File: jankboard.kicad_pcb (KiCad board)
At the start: 2 copper layers, 145.3 x 81 mm, 159 parts, among them J1 F31L-1A7H1-11030, J2 F31L-1A7H1-11030, J3 Conn_01x02, J4 Conn_01x02, J5 Conn_01x04_Pin, SW1 SW_Push_45deg, SW10 SW_Push_45deg, SW11 SW_Push_45deg, SW12 SW_Push_45deg, SW13 SW_Push_45deg, SW14 SW_Push_45deg, SW15 SW_Push_45deg, SW16 SW_Push_45deg, SW17 SW_Push_45deg, SW18 SW_Push_45deg, SW19 SW_Push_45deg, SW2 SW_Push_45deg, SW20 SW_Push_45deg, SW21 SW_Push_45deg, SW3 SW_Push_45deg, SW4 SW_Push_45deg, SW5 SW_Push_45deg, SW6 SW_Push_45deg, SW7 SW_Push_45deg, SW8 SW_Push_45deg, SW9 SW_Push_45deg, U1 nice_nano

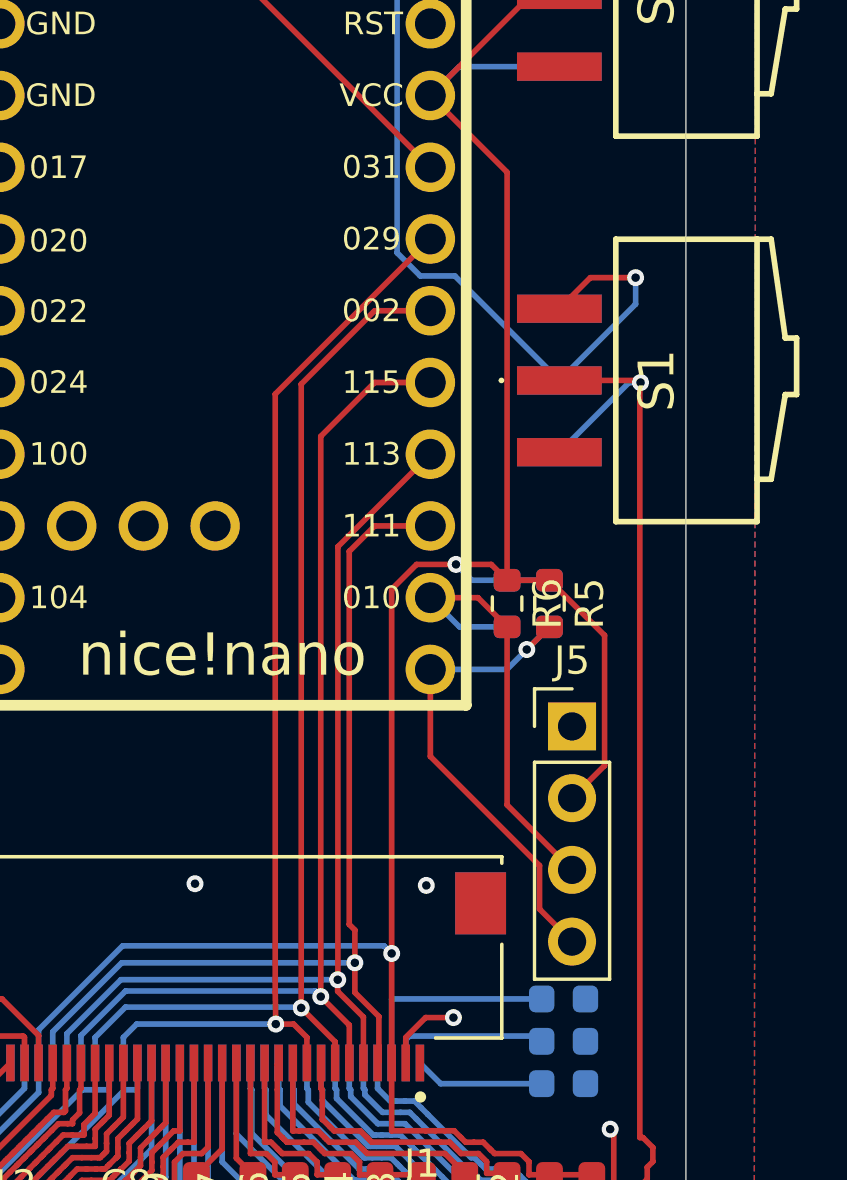
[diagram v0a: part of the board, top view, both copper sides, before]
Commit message: add models
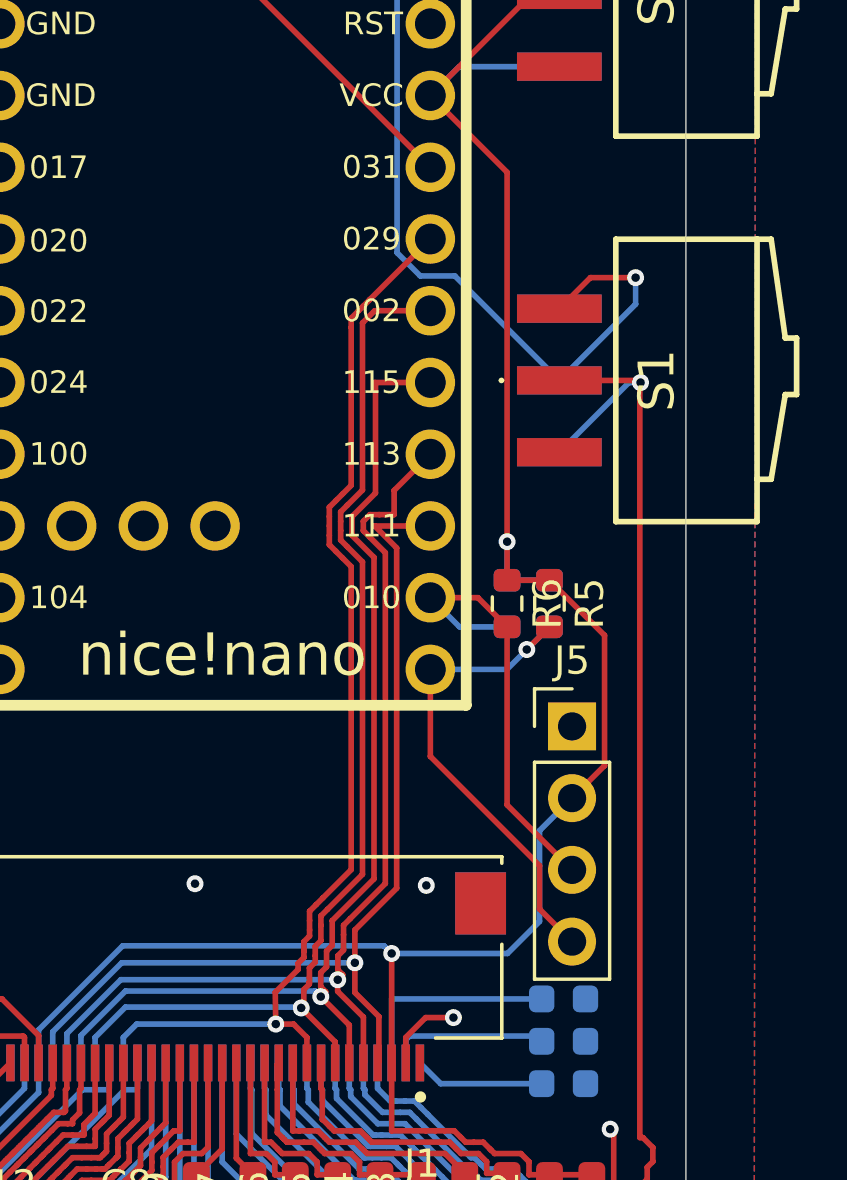
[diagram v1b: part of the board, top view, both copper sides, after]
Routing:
- net +3.3V: track 103.6 -> 95.9 mm
- net SCK: track 34.8 -> 36.1 mm
- net CS: track 37.5 -> 38.4 mm
- net DC: track 38.9 -> 39.6 mm
- net BUSY: track 38.8 -> 39.4 mm
